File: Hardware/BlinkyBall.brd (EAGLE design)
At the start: 3 parts, among them IC3 TINY13-20SSU

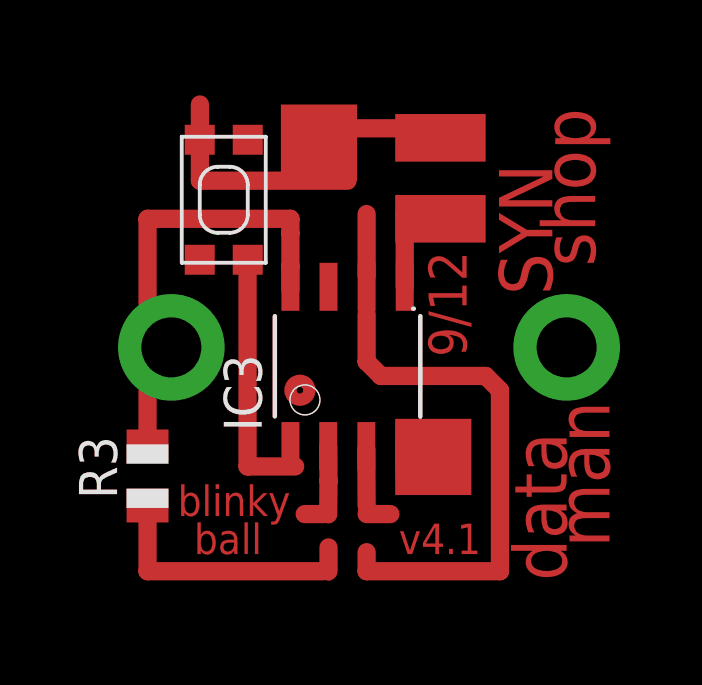
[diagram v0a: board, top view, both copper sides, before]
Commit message: tinkering
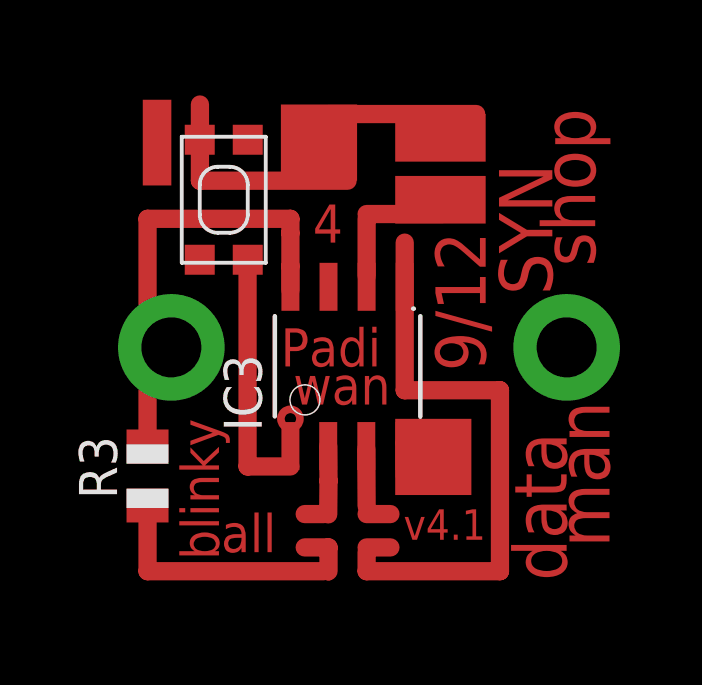
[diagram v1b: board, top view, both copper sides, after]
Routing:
- net N$25: track 4.65 -> 0.00 mm
- net S$5: track 0.00 -> 2.54 mm
- net S$11: track 17.5 -> 19.2 mm
- net S$13: track 0.79 -> 1.59 mm
- net S$6: track 0.00 -> 0.79 mm
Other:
- board text added: "4"
- board text added: "Padi"
- board text added: "all"
- board text added: "wan"
- board text removed: "ball"
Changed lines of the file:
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@@
 <board>
 <plain>
-<circle x="8.41375" y="8.5725" radius="0.3175" width="0.4064" layer="1"/>
-<text x="13.97" y="9.68375" size="1.27" layer="1" rot="R90">9/12</text>
-<circle x="13.49375" y="14.12875" radius="0.3175" width="0.4064" layer="16"/>
+<circle x="8.09625" y="7.62" radius="0.3175" width="0.254" layer="1"/>
+<text x="14.605" y="9.2075" size="1.6764" layer="1" rot="R90">9/12</text>
+<circle x="13.17625" y="14.76375" radius="0.3175" width="0.4064" layer="16"/>
 <rectangle x1="7.77875" y1="15.5575" x2="10.31875" y2="18.0975" layer="1"/>
 <rectangle x1="11.58875" y1="5.08" x2="14.12875" y2="7.62" layer="1"/>
 <rectangle x1="11.58875" y1="16.1925" x2="14.605" y2="17.78" layer="1"/>
-<rectangle x1="11.58875" y1="13.49375" x2="14.605" y2="15.08125" layer="1"/>
+<rectangle x1="11.58875" y1="14.12875" x2="14.605" y2="15.71625" layer="1"/>
 <text x="16.8275" y="11.7475" size="1.778" layer="1" rot="R90">SYN</text>
 <text x="18.7325" y="3.33375" size="1.778" layer="1" rot="R90">man</text>
-<text x="8.09625" y="5.3975" size="1.016" layer="1" rot="R180">blinky</text>
-<text x="7.14375" y="4.1275" size="1.016" layer="1" rot="R180">ball</text>
-<text x="14.44625" y="4.1275" size="1.016" layer="1" rot="R180">v4.1</text>
+<text x="4.445" y="7.62" size="1.27" layer="1" rot="R270">blinky</text>
+<text x="7.62" y="4.445" size="1.27" layer="1" rot="R180">all</text>
+<text x="14.605" y="4.60375" size="1.016" layer="1" rot="R180">v4.1</text>
 <text x="18.25625" y="12.7" size="1.778" layer="1" rot="R90">shop</text>
 <text x="17.30375" y="2.2225" size="1.778" layer="1" rot="R90">data</text>
+<text x="11.1125" y="10.63625" size="1.27" layer="1" rot="R180">Padi</text>
+<text x="11.43" y="9.36625" size="1.27" layer="1" rot="R180">wan</text>
+<text x="9.8425" y="14.76375" size="1.27" layer="1" rot="R180">4</text>
+<rectangle x1="3.175" y1="15.39875" x2="4.1275" y2="18.25625" layer="1"/>
 </plain>
 <attributes>
@@
 <signal name="N$25">
 <contactref element="IC3" pad="5"/>
-<wire x1="11.90625" y1="12.02025" x2="11.90625" y2="14.44625" width="0.6096" layer="1"/>
-<wire x1="11.90625" y1="14.44625" x2="14.12875" y2="14.44625" width="0.6096" layer="1"/>
+<wire x1="11.90625" y1="12.02025" x2="11.90625" y2="14.2875" width="0" layer="19" extent="1-16"/>
+<wire x1="11.90625" y1="14.2875" x2="14.12875" y2="14.44625" width="0" layer="19" extent="1-16"/>
 </signal>
 <signal name="N$26">
@@
 <signal name="S$2">
 <wire x1="10.63625" y1="4.445" x2="11.43" y2="4.445" width="0.6096" layer="1"/>
-<wire x1="9.36625" y1="17.30375" x2="14.2875" y2="17.30375" width="0.6096" layer="1"/>
+<wire x1="9.36625" y1="17.78" x2="14.2875" y2="17.78" width="0.6096" layer="1"/>
 </signal>
 <signal name="S$3">
@@
 <signal name="S$7">
 <wire x1="6.6675" y1="12.85875" x2="6.6675" y2="6.0325" width="0.6096" layer="1"/>
-<wire x1="6.6675" y1="6.0325" x2="8.255" y2="6.0325" width="0.6096" layer="1"/>
+<wire x1="6.6675" y1="6.0325" x2="8.09625" y2="6.0325" width="0.6096" layer="1"/>
 </signal>
 <signal name="S$10">
@@
 </signal>
 <signal name="S$11">
-<wire x1="10.63625" y1="11.1125" x2="10.63625" y2="9.525" width="0.6096" layer="1"/>
-<wire x1="10.63625" y1="9.525" x2="11.1125" y2="9.04875" width="0.6096" layer="1"/>
+<wire x1="11.90625" y1="13.49375" x2="11.90625" y2="8.5725" width="0.6096" layer="1"/>
 <wire x1="15.08125" y1="8.5725" x2="15.08125" y2="2.54" width="0.6096" layer="1"/>
 <wire x1="15.08125" y1="2.54" x2="10.63625" y2="2.54" width="0.6096" layer="1"/>
-<wire x1="11.1125" y1="9.04875" x2="14.605" y2="9.04875" width="0.6096" layer="1"/>
-<wire x1="14.605" y1="9.04875" x2="15.08125" y2="8.5725" width="0.6096" layer="1"/>
+<wire x1="11.90625" y1="8.5725" x2="15.08125" y2="8.5725" width="0.6096" layer="1"/>
 <wire x1="10.63625" y1="2.54" x2="10.63625" y2="3.175" width="0.6096" layer="1"/>
 </signal>
 <signal name="S$12">
-<wire x1="10.63625" y1="12.3825" x2="10.63625" y2="14.44625" width="0.6096" layer="1"/>
+<wire x1="10.63625" y1="12.3825" x2="10.63625" y2="14.2875" width="0.6096" layer="1"/>
 </signal>
 <signal name="S$8">
@@
 <signal name="S$13">
 <wire x1="9.36625" y1="2.54" x2="9.36625" y2="3.33375" width="0.6096" layer="1"/>
+<wire x1="9.36625" y1="3.33375" x2="8.5725" y2="3.33375" width="0.6096" layer="1"/>
 </signal>
 <signal name="S$1">
@@
 <wire x1="5.08" y1="15.5575" x2="5.08" y2="18.0975" width="0.6096" layer="1"/>
 </signal>
+<signal name="S$5">
+<wire x1="10.63625" y1="14.44625" x2="13.17625" y2="14.44625" width="0.6096" layer="1"/>
+</signal>
+<signal name="S$6">
+<wire x1="10.63625" y1="3.33375" x2="11.43" y2="3.33375" width="0.6096" layer="1"/>
+</signal>
 </signals>
